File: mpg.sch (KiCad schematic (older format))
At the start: 47 parts, among them J1 DB25_Male_MountingHoles, J2 Conn_01x04_Male, J3 Conn_01x03_Male, J4 Conn_01x02_Male, J5 RJ45_Shielded, Q1 BC847, Q2 BC847, Q3 BC847, Q4 BC847, Q5 BC847, SW1 SW_Push, U1 LD2981ABU33TR, U2 STM32G431K6Tx, U3 SN65HVD230, U4 ESDCAN24-2BLY, Y1 8MHz

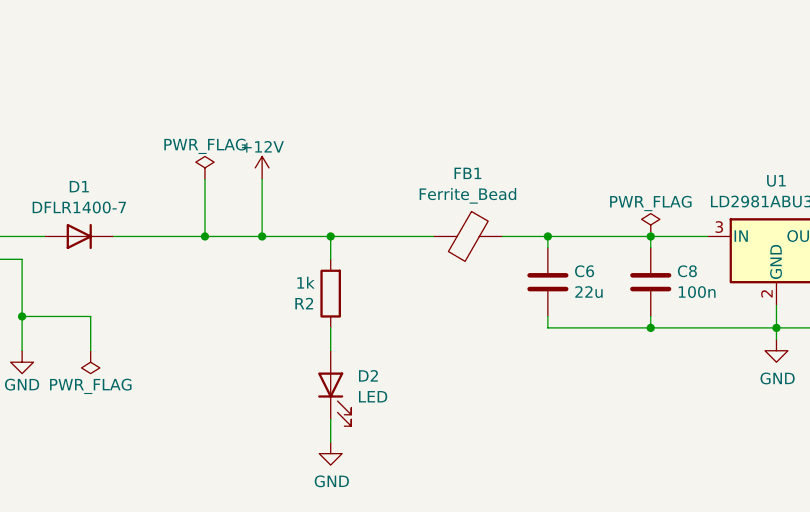
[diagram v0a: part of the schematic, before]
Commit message: Minor adjustments.
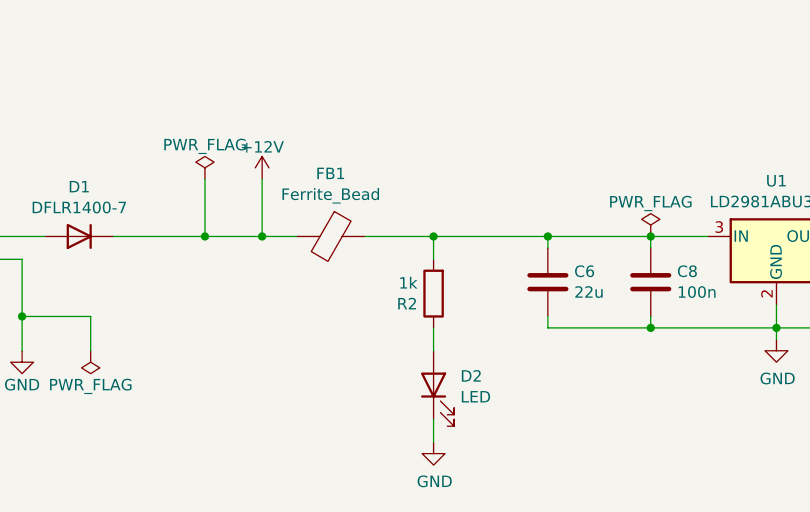
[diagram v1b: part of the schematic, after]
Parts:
- J4: footprint Connector_PinHeader_2.54mm:PinHeader_1x01_P2.54mm_Vertical -> Connector_PinHeader_2.54mm:PinHeader_1x02_P2.54mm_Vertical
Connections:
- net +12V: no longer R2.2
- net at C6.1, C8.1, FB1.1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: now also R2.2
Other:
- moved on the sheet: D2, FB1, R2
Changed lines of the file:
@@
 L Device:LED D?
 U 1 1 6017CAFF
-P 5300 10350
+P 5750 10350
 AR Path="/5F2EFD7F/6017CAFF" Ref="D?"  Part="1"
 AR Path="/6017CAFF" Ref="D2"  Part="1"
@@
 AR Path="/61500A32/6017CAFF" Ref="D?"  Part="1"
 AR Path="/60152FAB/6017CAFF" Ref="D?"  Part="1"
-F 0 "D2" V 5338 10233 50  0000 R CNN
-F 1 "LED" V 5247 10233 50  0000 R CNN
-F 2 "LED_SMD:LED_0603_1608Metric_Castellated" H 5300 10350 50  0001 C CNN
-F 3 "~" H 5300 10350 50  0001 C CNN
-	1    5300 10350
+F 0 "D2" V 5788 10233 50  0000 R CNN
+F 1 "LED" V 5697 10233 50  0000 R CNN
+F 2 "LED_SMD:LED_0603_1608Metric_Castellated" H 5750 10350 50  0001 C CNN
+F 3 "~" H 5750 10350 50  0001 C CNN
+	1    5750 10350
 	0    -1   -1   0
 $EndComp
@@
 L Device:R R?
 U 1 1 6017CB05
-P 5300 9950
+P 5750 9950
 AR Path="/5F2EFD7F/6017CB05" Ref="R?"  Part="1"
 AR Path="/6017CB05" Ref="R2"  Part="1"
@@
 AR Path="/61500A32/6017CB05" Ref="R?"  Part="1"
 AR Path="/60152FAB/6017CB05" Ref="R?"  Part="1"
-F 0 "R2" H 5370 9996 50  0000 L CNN
-F 1 "1k" H 5370 9905 50  0000 L CNN
-F 2 "Resistor_SMD:R_0603_1608Metric" V 5230 9950 50  0001 C CNN
-F 3 "~" H 5300 9950 50  0001 C CNN
-	1    5300 9950
+F 0 "R2" H 5820 9996 50  0000 L CNN
+F 1 "1k" H 5820 9905 50  0000 L CNN
+F 2 "Resistor_SMD:R_0603_1608Metric" V 5680 9950 50  0001 C CNN
+F 3 "~" H 5750 9950 50  0001 C CNN
+	1    5750 9950
 	-1   0    0    1
 $EndComp
@@
 L power:GND #PWR?
 U 1 1 6017CB0B
-P 5300 10600
+P 5750 10600
 AR Path="/5F2EFD7F/6017CB0B" Ref="#PWR?"  Part="1"
 AR Path="/6017CB0B" Ref="#PWR011"  Part="1"
@@
 AR Path="/61500A32/6017CB0B" Ref="#PWR?"  Part="1"
 AR Path="/60152FAB/6017CB0B" Ref="#PWR?"  Part="1"
-F 0 "#PWR011" H 5300 10350 50  0001 C CNN
-F 1 "GND" H 5305 10427 50  0000 C CNN
-F 2 "" H 5300 10600 50  0001 C CNN
-F 3 "" H 5300 10600 50  0001 C CNN
-	1    5300 10600
+F 0 "#PWR011" H 5750 10350 50  0001 C CNN
+F 1 "GND" H 5755 10427 50  0000 C CNN
+F 2 "" H 5750 10600 50  0001 C CNN
+F 3 "" H 5750 10600 50  0001 C CNN
+	1    5750 10600
 	1    0    0    -1
 $EndComp
@@
 $EndComp
 Wire Wire Line
-	6050 9700 6250 9700
+	5450 9700 5750 9700
 $Comp
 L Device:Ferrite_Bead FB?
 U 1 1 6017CB65
-P 5900 9700
+P 5300 9700
 AR Path="/5F2EFD7F/6017CB65" Ref="FB?"  Part="1"
 AR Path="/6017CB65" Ref="FB1"  Part="1"
@@
 AR Path="/61500A32/6017CB65" Ref="FB?"  Part="1"
 AR Path="/60152FAB/6017CB65" Ref="FB?"  Part="1"
-F 0 "FB1" V 5626 9700 50  0000 C CNN
-F 1 "Ferrite_Bead" V 5717 9700 50  0000 C CNN
-F 2 "Inductor_SMD:L_0603_1608Metric" V 5830 9700 50  0001 C CNN
-F 3 "~" H 5900 9700 50  0001 C CNN
-	1    5900 9700
+F 0 "FB1" V 5026 9700 50  0000 C CNN
+F 1 "Ferrite_Bead" V 5117 9700 50  0000 C CNN
+F 2 "Inductor_SMD:L_0603_1608Metric" V 5230 9700 50  0001 C CNN
+F 3 "~" H 5300 9700 50  0001 C CNN
+	1    5300 9700
 	0    1    1    0
 $EndComp
@@
 	5000 9700 4750 9700
 Wire Wire Line
-	5300 10500 5300 10600
-Wire Wire Line
-	5300 10100 5300 10200
+	5750 10500 5750 10600
+Wire Wire Line
+	5750 10100 5750 10200
 Wire Wire Line
 	3650 9700 4050 9700
@@
 Wire Wire Line
 	3950 10050 3950 10200
-Wire Wire Line
-	5000 9700 5300 9700
-Wire Wire Line
-	5300 9800 5300 9700
-Connection ~ 5300 9700
-Wire Wire Line
-	5300 9700 5750 9700
 $Comp
 L power:+3.3V #PWR020
@@
 F 0 "J4" H 10622 4474 50  0000 R CNN
 F 1 "Conn_01x02_Male" H 10622 4383 50  0000 R CNN
-F 2 "Connector_PinHeader_2.54mm:PinHeader_1x01_P2.54mm_Vertical" H 10650 4500 50  0001 C CNN
+F 2 "Connector_PinHeader_2.54mm:PinHeader_1x02_P2.54mm_Vertical" H 10650 4500 50  0001 C CNN
 F 3 "~" H 10650 4500 50  0001 C CNN
 	1    10650 4500
@@
 Wire Wire Line
 	3900 2400 4000 2400
+Wire Wire Line
+	5000 9700 5150 9700
+Wire Wire Line
+	5750 9800 5750 9700
+Connection ~ 5750 9700
+Wire Wire Line
+	5750 9700 6250 9700
 $EndSCHEMATC
